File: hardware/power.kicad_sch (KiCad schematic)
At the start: 47 parts, among them J8 USB_C_Receptacle_USB2.0_16P, Q1 AO3400A, U10 EL817S1C, U12 USBLC6-2SC6, U2 IP5306, U7 AOZ1280CI

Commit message: Removed old readme, added files.
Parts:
- C1: MPN CL05B104KB54PNC -> CL05B105KQ5NQNC
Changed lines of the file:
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@@
 			)
 		)
-		(property "MPN" "CL05B104KB54PNC"
+		(property "MPN" "CL05B105KQ5NQNC"
 			(at 236.22 36.83 0)
 			(effects

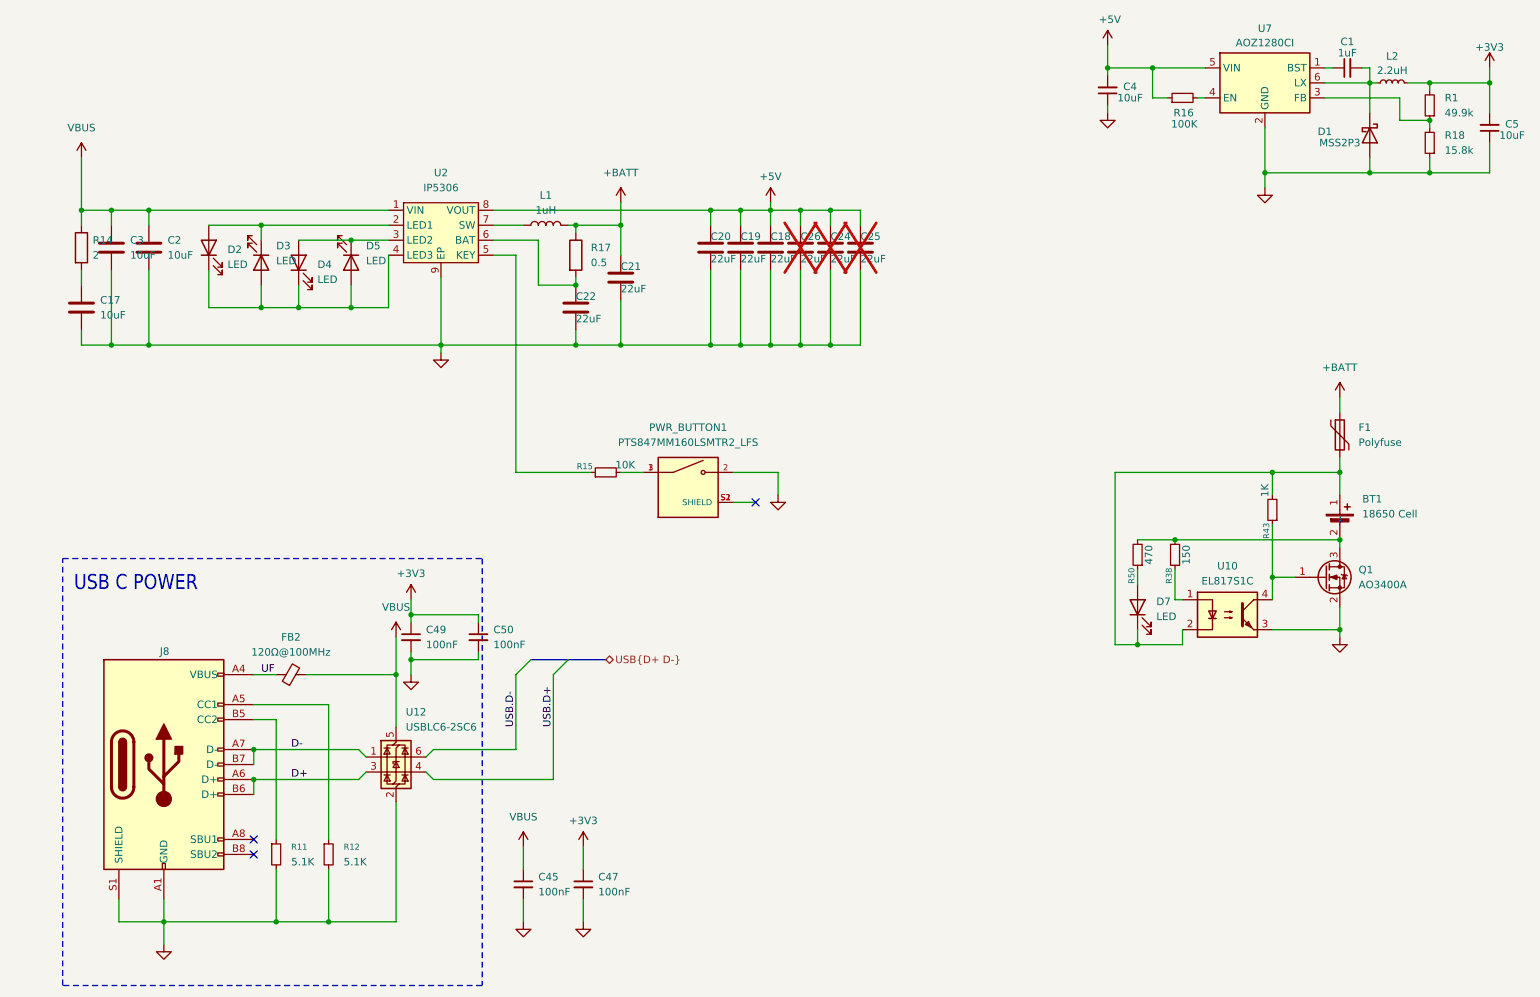
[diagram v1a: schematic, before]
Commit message: R1.0 released.
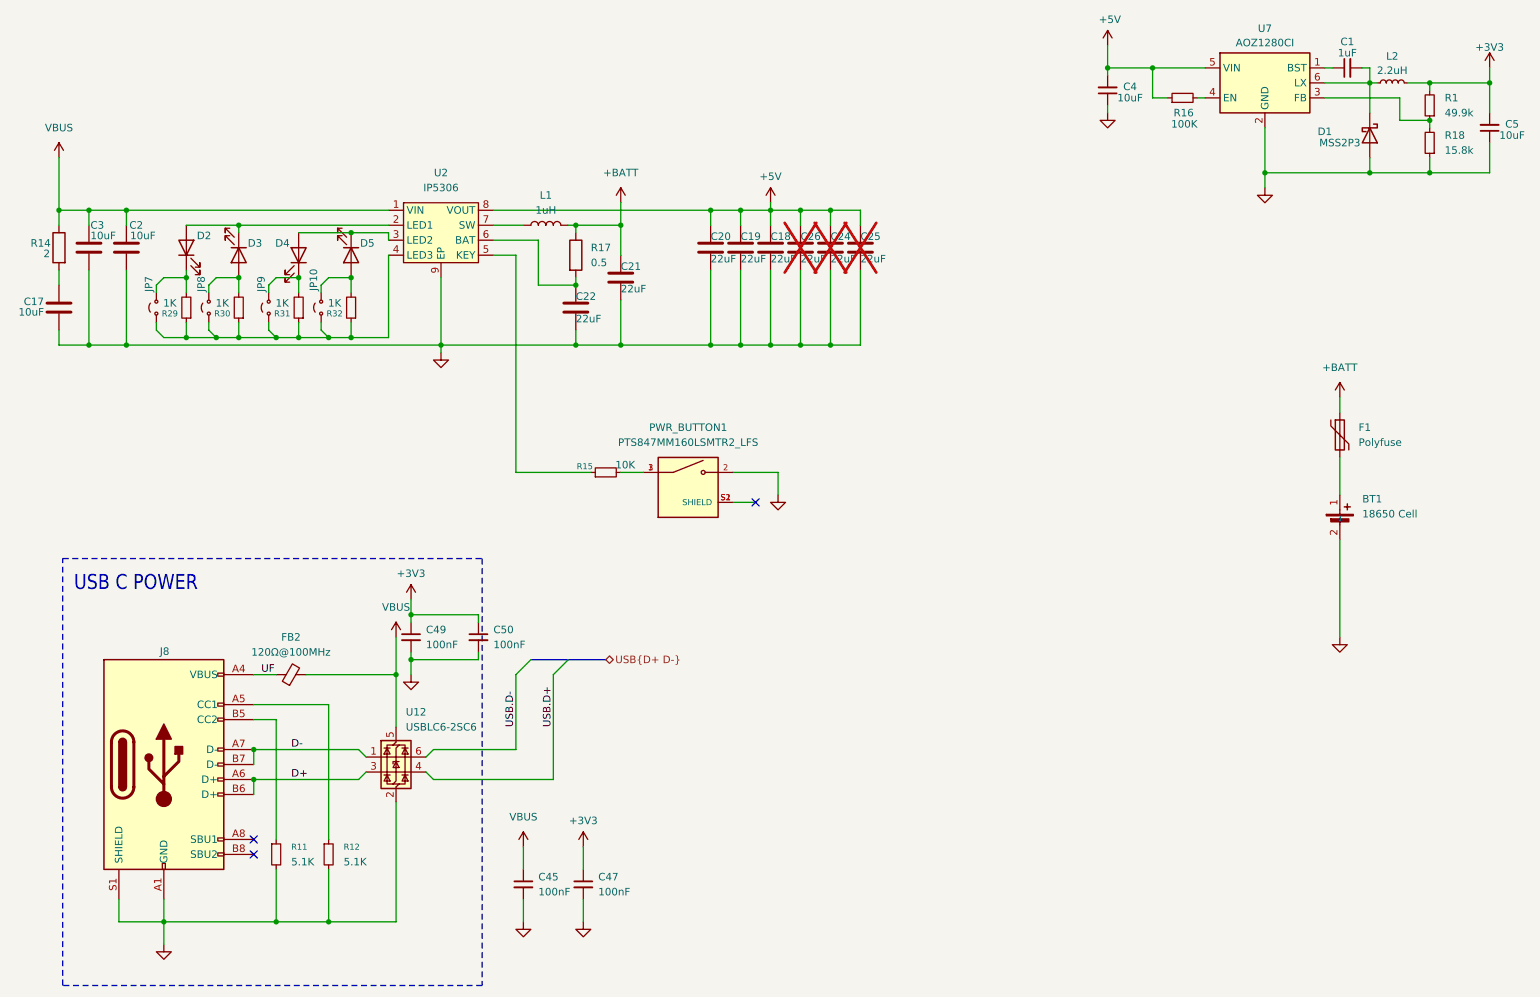
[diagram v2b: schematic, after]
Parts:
- removed D7: LED, LED_SMD:LED_0603_1608Metric, symbol Device:LED
- removed Q1: AO3400A, Package_TO_SOT_SMD:SOT-23, symbol Transistor_FET:AO3400A
- removed R38: 150, Resistor_SMD:R_0402_1005Metric, symbol Device:R_Small
- removed R43: 1K, Resistor_SMD:R_0402_1005Metric, symbol Device:R_Small
- removed R50: 470, Resistor_SMD:R_0402_1005Metric, symbol Device:R_Small
- removed U10: EL817S1C, EL817:SOIC254P1030X390-4N, symbol Isolator:EL817
- added JP10, JP7, JP8, JP9: Jumper_2_Small_Open, Jumper:SolderJumper-2_P1.3mm_Open_RoundedPad1.0x1.5mm, symbol Jumper:Jumper_2_Small_Open
- added R29, R30, R31, R32: 1K, Resistor_SMD:R_0402_1005Metric, symbol Device:R_Small
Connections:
- net GND: now also BT1.2 (-)
- new net: D4.1 (K), JP9.2 (B), R31.2
- new net: JP10.1 (A), JP7.1 (A), JP8.1 (A), JP9.1 (A), R29.1, R30.1, R31.1, R32.1, U2.4 (LED3)
- new net: D5.2 (A), JP10.2 (B), R32.2
- new net: D2.1 (K), JP7.2 (B), R29.2
- new net: D3.2 (A), JP8.2 (B), R30.2
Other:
- moved on the sheet: C17, C2, C3, D2, D3, D4, D5, R14
